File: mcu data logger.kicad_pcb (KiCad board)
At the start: 2 copper layers, 50.6 x 31.6 mm, 29 parts, among them J1 Conn_01x04_Pin, J2 Conn_01x09_Pin, J3 Conn_01x04_Pin, J4 Conn_02x03_Odd_Even, U1 24LC1025, U2 DS1337S_, U3 24LC1025, U4 ATMEGA328P-AU, Y1 32.768 KHz, Y2 16 MHz

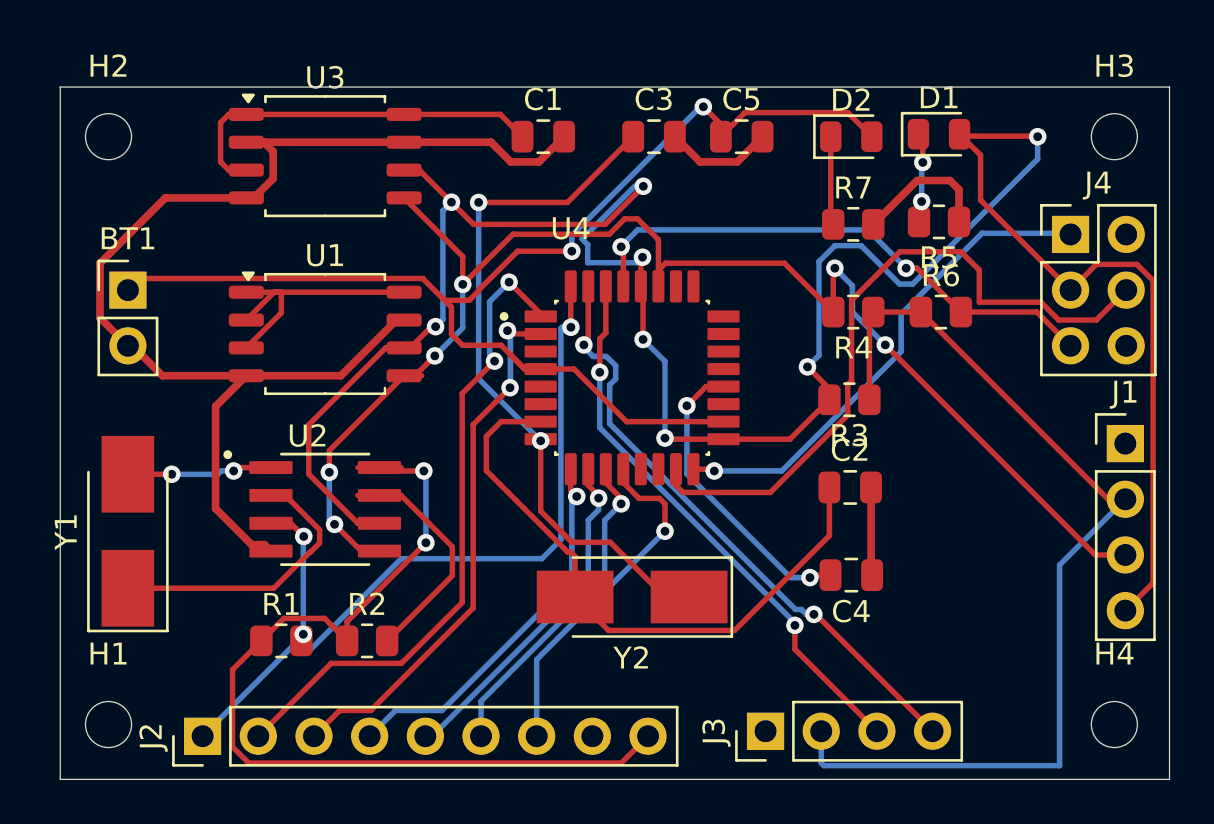
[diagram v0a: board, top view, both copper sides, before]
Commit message: completed routing
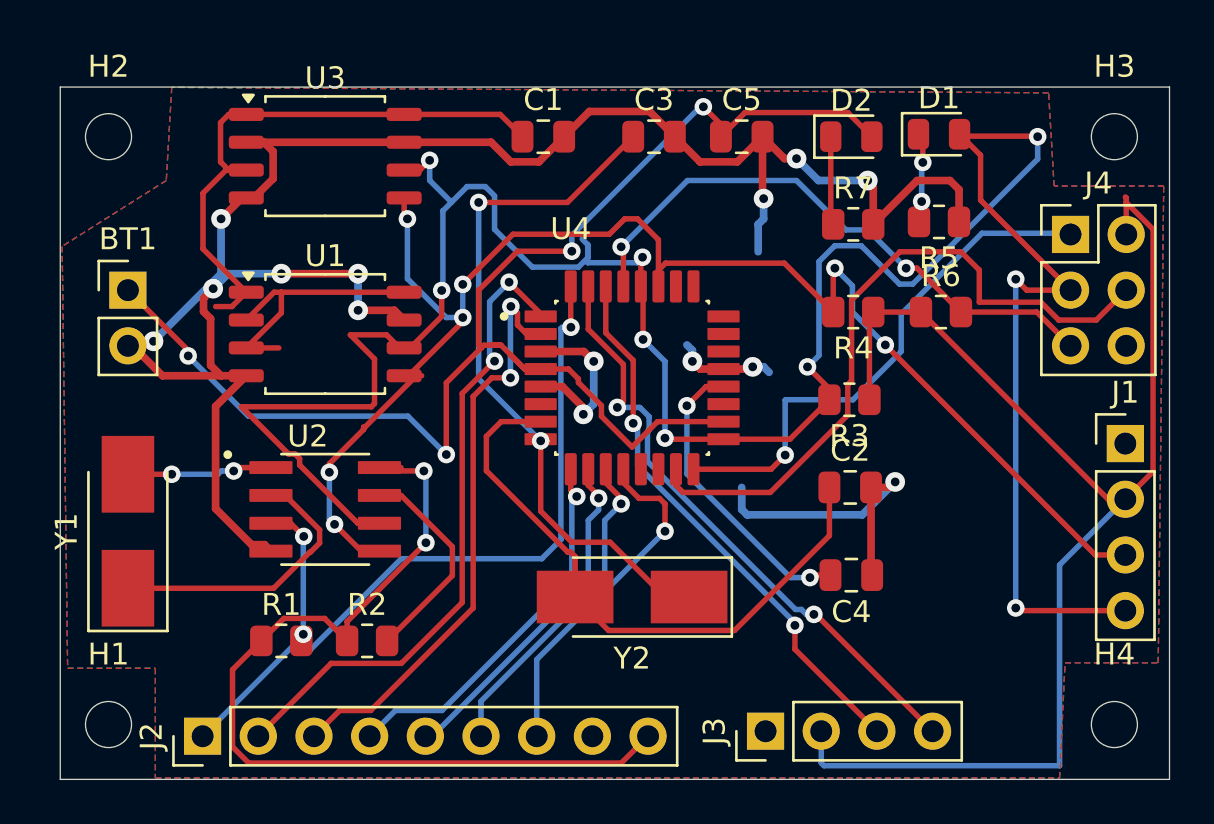
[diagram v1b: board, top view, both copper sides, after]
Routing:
- net GND: track 71.6 -> 118.5 mm, vias 0 -> 14
- net /VCC: track 118.1 -> 142.7 mm
- net /SCK: track 111.7 -> 119.9 mm, vias 8 -> 9
- net Net-(BT1-+): track 57.9 -> 65.8 mm, vias 2 -> 4
- net /SDA: track 65.4 -> 68.1 mm, vias 6 -> 7
- net /D4: track 24.7 -> 26.8 mm
- net /RESET: track 24.9 -> 26.7 mm
- net /MISO: track 22.8 -> 24.2 mm
- net Net-(U2-SQW/~INT): track 10.8 -> 9.82 mm
- net /RX: track 26.3 -> 25.4 mm
- net /TX: track 27.6 -> 28.1 mm
- added copper zone on F.Cu, net /VCC
- added copper zone on B.Cu, net GND
